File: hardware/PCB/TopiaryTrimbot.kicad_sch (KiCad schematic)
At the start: 4 parts

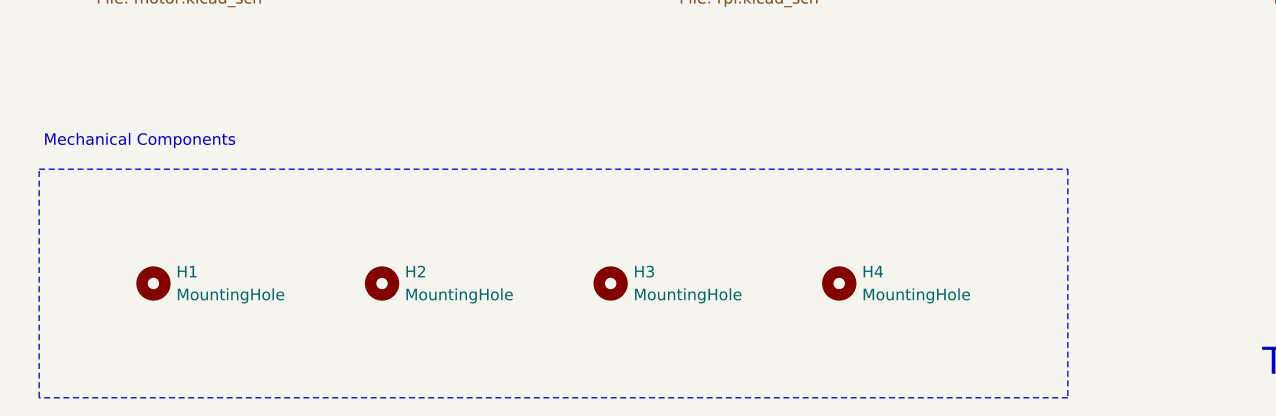
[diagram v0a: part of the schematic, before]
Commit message: Final changes before submission to website
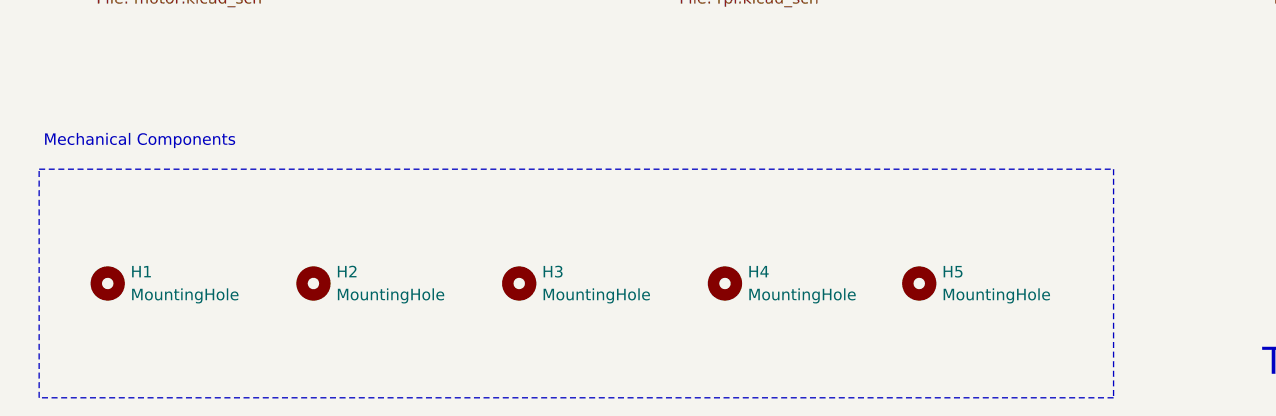
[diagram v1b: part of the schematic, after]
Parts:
- added H5: MountingHole, MountingHole:MountingHole_3.2mm_M3_Pad_TopBottom, symbol Mechanical:MountingHole
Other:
- moved on the sheet: H1, H2, H3, H4
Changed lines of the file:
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@@
 	(rectangle
 		(start 50.8 152.4)
-		(end 165.1 177.8)
+		(end 170.18 177.8)
 		(stroke
 			(width 0)
@@
 	(symbol
 		(lib_id "Mechanical:MountingHole")
-		(at 139.7 165.1 0)
+		(at 127 165.1 0)
 		(unit 1)
 		(exclude_from_sim no)
@@
 		(fields_autoplaced yes)
 		(property "Reference" "H4"
-			(at 142.24 163.8299 0)
+			(at 129.54 163.8299 0)
 			(effects
 				(font
@@
 		)
 		(property "Value" "MountingHole"
-			(at 142.24 166.3699 0)
+			(at 129.54 166.3699 0)
 			(effects
 				(font
@@
 		)
 		(property "Footprint" "MountingHole:MountingHole_3.2mm_M3_Pad_TopBottom"
-			(at 139.7 165.1 0)
+			(at 127 165.1 0)
 			(effects
 				(font
@@
 		)
 		(property "Datasheet" "~"
-			(at 139.7 165.1 0)
+			(at 127 165.1 0)
 			(effects
 				(font
@@
 		)
 		(property "Description" "Mounting Hole without connection"
-			(at 139.7 165.1 0)
+			(at 127 165.1 0)
 			(effects
 				(font
@@
 		)
 		(property "MANUFACTURER" "~"
-			(at 139.7 165.1 0)
+			(at 127 165.1 0)
 			(effects
 				(font
@@
 		)
 		(property "Manufacturer_Part_Number" "~"
-			(at 139.7 165.1 0)
+			(at 127 165.1 0)
 			(effects
 				(font
@@
 	(symbol
 		(lib_id "Mechanical:MountingHole")
-		(at 114.3 165.1 0)
+		(at 104.14 165.1 0)
 		(unit 1)
 		(exclude_from_sim no)
@@
 		(fields_autoplaced yes)
 		(property "Reference" "H3"
-			(at 116.84 163.8299 0)
+			(at 106.68 163.8299 0)
 			(effects
 				(font
@@
 		)
 		(property "Value" "MountingHole"
-			(at 116.84 166.3699 0)
+			(at 106.68 166.3699 0)
 			(effects
 				(font
@@
 		)
 		(property "Footprint" "MountingHole:MountingHole_3.2mm_M3_Pad_TopBottom"
-			(at 114.3 165.1 0)
+			(at 104.14 165.1 0)
 			(effects
 				(font
@@
 		)
 		(property "Datasheet" "~"
-			(at 114.3 165.1 0)
+			(at 104.14 165.1 0)
 			(effects
 				(font
@@
 		)
 		(property "Description" "Mounting Hole without connection"
-			(at 114.3 165.1 0)
+			(at 104.14 165.1 0)
 			(effects
 				(font
@@
 		)
 		(property "MANUFACTURER" "~"
-			(at 114.3 165.1 0)
+			(at 104.14 165.1 0)
 			(effects
 				(font
@@
 		)
 		(property "Manufacturer_Part_Number" "~"
-			(at 114.3 165.1 0)
+			(at 104.14 165.1 0)
 			(effects
 				(font
@@
 	(symbol
 		(lib_id "Mechanical:MountingHole")
-		(at 63.5 165.1 0)
+		(at 58.42 165.1 0)
 		(unit 1)
 		(exclude_from_sim no)
@@
 		(fields_autoplaced yes)
 		(property "Reference" "H1"
-			(at 66.04 163.8299 0)
+			(at 60.96 163.8299 0)
 			(effects
 				(font
@@
 		)
 		(property "Value" "MountingHole"
-			(at 66.04 166.3699 0)
+			(at 60.96 166.3699 0)
 			(effects
 				(font
@@
 		)
 		(property "Footprint" "MountingHole:MountingHole_3.2mm_M3_Pad_TopBottom"
-			(at 63.5 165.1 0)
+			(at 58.42 165.1 0)
 			(effects
 				(font
@@
 		)
 		(property "Datasheet" "~"
-			(at 63.5 165.1 0)
+			(at 58.42 165.1 0)
 			(effects
 				(font
@@
 		)
 		(property "Description" "Mounting Hole without connection"
-			(at 63.5 165.1 0)
+			(at 58.42 165.1 0)
 			(effects
 				(font
@@
 		)
 		(property "MANUFACTURER" "~"
-			(at 63.5 165.1 0)
+			(at 58.42 165.1 0)
 			(effects
 				(font
@@
 		)
 		(property "Manufacturer_Part_Number" "~"
-			(at 63.5 165.1 0)
+			(at 58.42 165.1 0)
 			(effects
 				(font
@@
 	(symbol
 		(lib_id "Mechanical:MountingHole")
-		(at 88.9 165.1 0)
+		(at 148.59 165.1 0)
+		(unit 1)
+		(exclude_from_sim no)
+		(in_bom no)
+		(on_board yes)
+		(dnp no)
+		(fields_autoplaced yes)
+		(property "Reference" "H5"
+			(at 151.13 163.8299 0)
+			(effects
+				(font
+					(size 1.27 1.27)
+				)
+				(justify left)
+			)
+		)
+		(property "Value" "MountingHole"
+			(at 151.13 166.3699 0)
+			(effects
+				(font
+					(size 1.27 1.27)
+				)
+				(justify left)
+			)
+		)
+		(property "Footprint" "MountingHole:MountingHole_3.2mm_M3_Pad_TopBottom"
+			(at 148.59 165.1 0)
+			(effects
+				(font
+					(size 1.27 1.27)
+				)
+				(hide yes)
+			)
+		)
+		(property "Datasheet" "~"
+			(at 148.59 165.1 0)
+			(effects
+				(font
+					(size 1.27 1.27)
+				)
+				(hide yes)
+			)
+		)
+		(property "Description" "Mounting Hole without connection"
+			(at 148.59 165.1 0)
+			(effects
+				(font
+					(size 1.27 1.27)
+				)
+				(hide yes)
+			)
+		)
+		(property "MANUFACTURER" "~"
+			(at 148.59 165.1 0)
+			(effects
+				(font
+					(size 1.27 1.27)
+				)
+				(hide yes)
+			)
+		)
+		(property "Manufacturer_Part_Number" "~"
+			(at 148.59 165.1 0)
+			(effects
+				(font
+					(size 1.27 1.27)
+				)
+				(hide yes)
+			)
+		)
+		(instances
+			(project "TopiaryTrimbot"
+				(path "/2826ff7c-9767-4078-8ea2-1cd3a432abf3"
+					(reference "H5")
+					(unit 1)
+				)
+			)
+		)
+	)
+	(symbol
+		(lib_id "Mechanical:MountingHole")
+		(at 81.28 165.1 0)
 		(unit 1)
 		(exclude_from_sim no)
@@
 		(fields_autoplaced yes)
 		(property "Reference" "H2"
-			(at 91.44 163.8299 0)
+			(at 83.82 163.8299 0)
 			(effects
 				(font
@@
 		)
 		(property "Value" "MountingHole"
-			(at 91.44 166.3699 0)
+			(at 83.82 166.3699 0)
 			(effects
 				(font
@@
 		)
 		(property "Footprint" "MountingHole:MountingHole_3.2mm_M3_Pad_TopBottom"
-			(at 88.9 165.1 0)
+			(at 81.28 165.1 0)
 			(effects
 				(font
@@
 		)
 		(property "Datasheet" "~"
-			(at 88.9 165.1 0)
+			(at 81.28 165.1 0)
 			(effects
 				(font
@@
 		)
 		(property "Description" "Mounting Hole without connection"
-			(at 88.9 165.1 0)
+			(at 81.28 165.1 0)
 			(effects
 				(font
@@
 		)
 		(property "MANUFACTURER" "~"
-			(at 88.9 165.1 0)
+			(at 81.28 165.1 0)
 			(effects
 				(font
@@
 		)
 		(property "Manufacturer_Part_Number" "~"
-			(at 88.9 165.1 0)
-			(effects
-				(font
+			(at 81.28 165.1 0)
+			(effects
+				(font
